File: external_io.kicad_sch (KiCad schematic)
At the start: 13 parts, among them J1 UJ20-C-H-G-SMT-1-P16-TR, J3 Conn_01x02_Socket, J4 Conn_01x04_Socket, J5 Conn_01x03_Socket, J6 Conn_01x03_Socket, J7 Conn_01x03_Socket, U1 USBLC6-2SC6, U2 USBLC6-2SC6

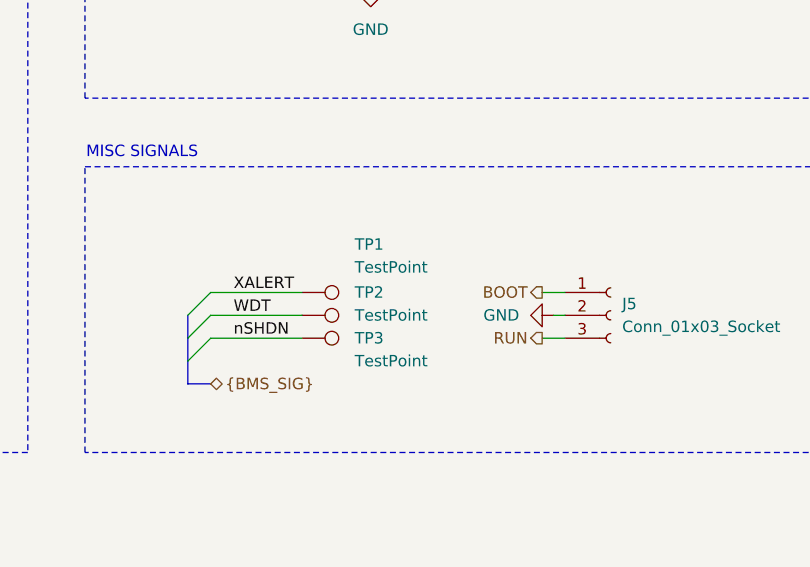
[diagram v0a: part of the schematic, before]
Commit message: Did a lot of routing
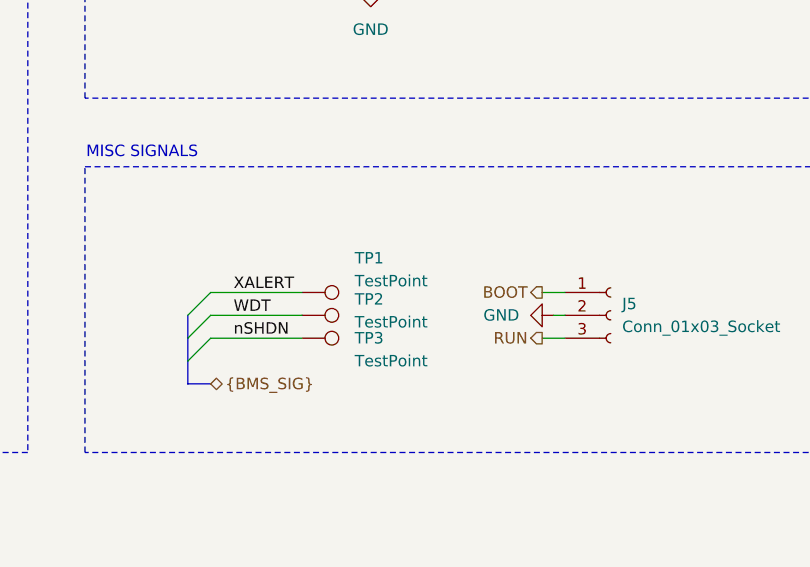
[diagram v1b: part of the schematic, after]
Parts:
- TP1, TP2, TP3: footprint TestPoint:TestPoint_Keystone_5015_Micro_Mini -> _BMS:Harwin TP
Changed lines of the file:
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@@
 			)
 		)
-		(property "Footprint" "TestPoint:TestPoint_Keystone_5015_Micro_Mini"
+		(property "Footprint" "_BMS:Harwin TP"
 			(at 118.11 87.63 0)
 			(effects
@@
 		(dnp no)
 		(property "Reference" "TP2"
-			(at 123.952 77.47 90)
+			(at 123.952 78.232 90)
 			(effects
 				(font
@@
 		)
 		(property "Value" "TestPoint"
-			(at 123.952 80.01 90)
+			(at 123.952 80.772 90)
 			(effects
 				(font
@@
 			)
 		)
-		(property "Footprint" "TestPoint:TestPoint_Keystone_5015_Micro_Mini"
+		(property "Footprint" "_BMS:Harwin TP"
 			(at 118.11 85.09 0)
 			(effects
@@
 	)
 	(symbol
-		(lib_id "Connector:TestPoint")
-		(at 118.11 77.47 270)
-		(unit 1)
-		(exclude_from_sim no)
-		(in_bom yes)
-		(on_board yes)
-		(dnp no)
-		(property "Reference" "TP1"
-			(at 123.952 72.136 90)
-			(effects
-				(font
-					(size 1.27 1.27)
-				)
-				(justify left)
-			)
-		)
-		(property "Value" "TestPoint"
-			(at 123.952 74.676 90)
-			(effects
-				(font
-					(size 1.27 1.27)
-				)
-				(justify left)
-			)
-		)
-		(property "Footprint" "TestPoint:TestPoint_Keystone_5015_Micro_Mini"
-			(at 118.11 82.55 0)
-			(effects
-				(font
-					(size 1.27 1.27)
-				)
-				(hide yes)
-			)
-		)
-		(property "Datasheet" "~"
-			(at 118.11 82.55 0)
-			(effects
-				(font
-					(size 1.27 1.27)
-				)
-				(hide yes)
-			)
-		)
-		(property "Description" "test point"
-			(at 118.11 77.47 0)
-			(effects
-				(font
-					(size 1.27 1.27)
-				)
-				(hide yes)
-			)
-		)
-		(property "Mfr" ""
-			(at 118.11 77.47 0)
-			(effects
-				(font
-					(size 1.27 1.27)
-				)
-				(hide yes)
-			)
-		)
-		(property "Mfr P/N" ""
-			(at 118.11 77.47 0)
-			(effects
-				(font
-					(size 1.27 1.27)
-				)
-				(hide yes)
-			)
-		)
-		(property "Supplier_1" ""
-			(at 118.11 77.47 0)
-			(effects
-				(font
-					(size 1.27 1.27)
-				)
-				(hide yes)
-			)
-		)
-		(property "Supplier_1 P/N" ""
-			(at 118.11 77.47 0)
-			(effects
-				(font
-					(size 1.27 1.27)
-				)
-				(hide yes)
-			)
-		)
-		(property "Supplier_1 Unit Price" ""
-			(at 118.11 77.47 0)
-			(effects
-				(font
-					(size 1.27 1.27)
-				)
-				(hide yes)
-			)
-		)
-		(property "Supplier_1 Price @ Qty" ""
-			(at 118.11 77.47 0)
-			(effects
-				(font
-					(size 1.27 1.27)
-				)
-				(hide yes)
-			)
-		)
-		(property "Supplier_2" ""
-			(at 118.11 77.47 0)
-			(effects
-				(font
-					(size 1.27 1.27)
-				)
-				(hide yes)
-			)
-		)
-		(property "Supplier_2 P/N" ""
-			(at 118.11 77.47 0)
-			(effects
-				(font
-					(size 1.27 1.27)
-				)
-				(hide yes)
-			)
-		)
-		(property "Supplier_2 Unit Price" ""
-			(at 118.11 77.47 0)
-			(effects
-				(font
-					(size 1.27 1.27)
-				)
-				(hide yes)
-			)
-		)
-		(property "Supplier_2 Price @ Qty" ""
-			(at 118.11 77.47 0)
-			(effects
-				(font
-					(size 1.27 1.27)
-				)
-				(hide yes)
-			)
-		)
-		(pin "1"
-		)
-		(instances
-			(project ""
-				(path "/124184ba-5d68-4d9f-8da6-acc6720ab30b/93f9b420-7cce-46a9-9201-666f07a18f85/2982e12c-39cd-4158-a648-a90b7f6b527c"
-					(reference "TP1")
-					(unit 1)
-				)
-			)
-		)
-	)
-	(symbol
 		(lib_id "Connector:Conn_01x02_Socket")
 		(at 140.97 138.43 0)
@@
 					(unit 1)
 				)
+			)
+		)
+	)
+	(symbol
+		(lib_id "Connector:TestPoint")
+		(at 118.11 77.47 270)
+		(unit 1)
+		(exclude_from_sim no)
+		(in_bom yes)
+		(on_board yes)
+		(dnp no)
+		(property "Reference" "TP1"
+			(at 123.952 73.66 90)
+			(effects
+				(font
+					(size 1.27 1.27)
+				)
+				(justify left)
+			)
+		)
+		(property "Value" "TestPoint"
+			(at 123.952 76.2 90)
+			(effects
+				(font
+					(size 1.27 1.27)
+				)
+				(justify left)
+			)
+		)
+		(property "Footprint" "_BMS:Harwin TP"
+			(at 118.11 82.55 0)
+			(effects
+				(font
+					(size 1.27 1.27)
+				)
+				(hide yes)
+			)
+		)
+		(property "Datasheet" "~"
+			(at 118.11 82.55 0)
+			(effects
+				(font
+					(size 1.27 1.27)
+				)
+				(hide yes)
+			)
+		)
+		(property "Description" "test point"
+			(at 118.11 77.47 0)
+			(effects
+				(font
+					(size 1.27 1.27)
+				)
+				(hide yes)
+			)
+		)
+		(property "Mfr" ""
+			(at 118.11 77.47 0)
+			(effects
+				(font
+					(size 1.27 1.27)
+				)
+				(hide yes)
+			)
+		)
+		(property "Mfr P/N" ""
+			(at 118.11 77.47 0)
+			(effects
+				(font
+					(size 1.27 1.27)
+				)
+				(hide yes)
+			)
+		)
+		(property "Supplier_1" ""
+			(at 118.11 77.47 0)
+			(effects
+				(font
+					(size 1.27 1.27)
+				)
+				(hide yes)
+			)
+		)
+		(property "Supplier_1 P/N" ""
+			(at 118.11 77.47 0)
+			(effects
+				(font
+					(size 1.27 1.27)
+				)
+				(hide yes)
+			)
+		)
+		(property "Supplier_1 Unit Price" ""
+			(at 118.11 77.47 0)
+			(effects
+				(font
+					(size 1.27 1.27)
+				)
+				(hide yes)
+			)
+		)
+		(property "Supplier_1 Price @ Qty" ""
+			(at 118.11 77.47 0)
+			(effects
+				(font
+					(size 1.27 1.27)
+				)
+				(hide yes)
+			)
+		)
+		(property "Supplier_2" ""
+			(at 118.11 77.47 0)
+			(effects
+				(font
+					(size 1.27 1.27)
+				)
+				(hide yes)
+			)
+		)
+		(property "Supplier_2 P/N" ""
+			(at 118.11 77.47 0)
+			(effects
+				(font
+					(size 1.27 1.27)
+				)
+				(hide yes)
+			)
+		)
+		(property "Supplier_2 Unit Price" ""
+			(at 118.11 77.47 0)
+			(effects
+				(font
+					(size 1.27 1.27)
+				)
+				(hide yes)
+			)
+		)
+		(property "Supplier_2 Price @ Qty" ""
+			(at 118.11 77.47 0)
+			(effects
+				(font
+					(size 1.27 1.27)
+				)
+				(hide yes)
+			)
+		)
+		(pin "1"
+		)
+		(instances
+			(project "BMS"
+				(path "/124184ba-5d68-4d9f-8da6-acc6720ab30b/93f9b420-7cce-46a9-9201-666f07a18f85/2982e12c-39cd-4158-a648-a90b7f6b527c"
+					(reference "TP1")
+					(unit 1)
+				)

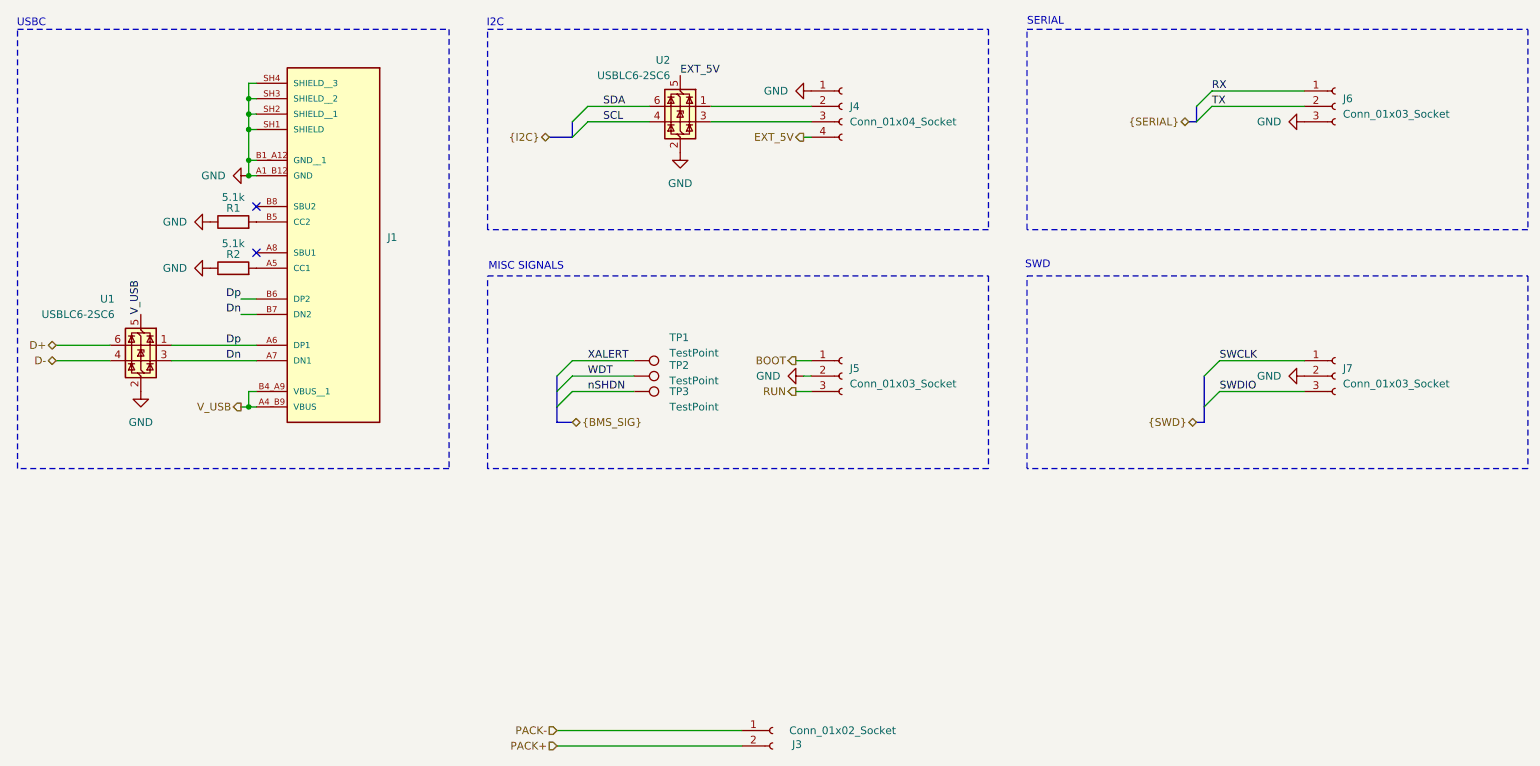
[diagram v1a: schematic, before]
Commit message: Pushing
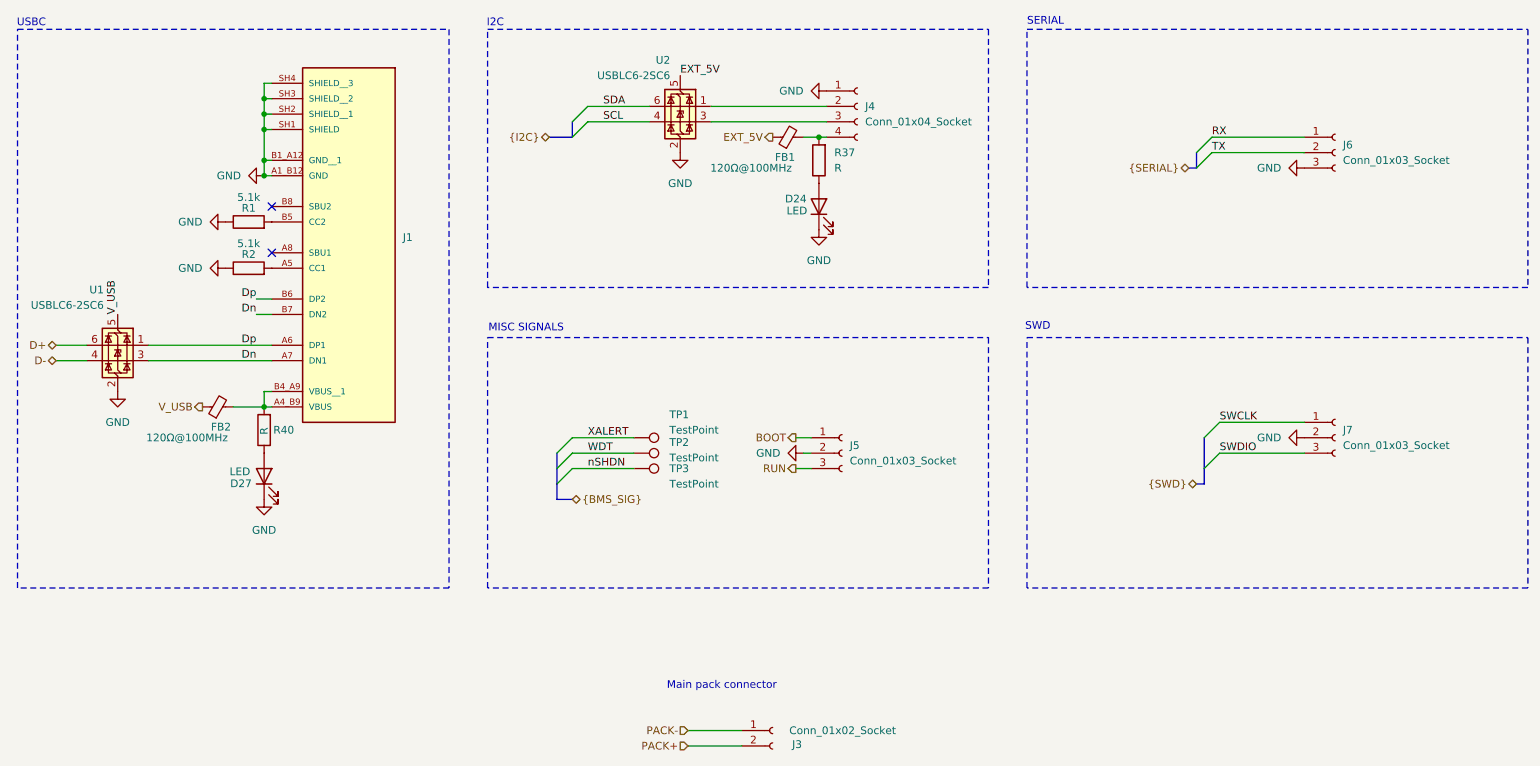
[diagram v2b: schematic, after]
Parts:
- added D24, D27: LED, symbol Device:LED
- added FB1, FB2: 120Ω@100MHz, Inductor_SMD:L_0603_1608Metric, symbol Device:FerriteBead_Small
- added R37, R40: R, symbol Device:R
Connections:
- net EXT_5V: now also FB1.1; no longer J4.4 (Pin_4)
- net GND: now also D24.1 (K), D27.1 (K)
- net V_USB: now also FB2.1; no longer J1.A4_B9 (VBUS), J1.B4_A9 (VBUS__1)
- new net: FB1.2, J4.4 (Pin_4), R37.2
- new net: FB2.2, J1.A4_B9 (VBUS), J1.B4_A9 (VBUS__1), R40.2
- new net: D24.2 (A), R37.1
- new net: D27.2 (A), R40.1
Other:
- note added: "Main pack connector"
- moved on the sheet: J1, J4, J5, J6, J7, R1, R2, TP1, TP2, TP3, U1
